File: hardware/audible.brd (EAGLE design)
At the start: 27.7 x 23.4 mm, 30 parts, among them IC1 LTC1966CMS8, J1 SQUALL_HEADER, J2 HIROSE-DF40C-10DP-0.4V, J3 HIROSE-DF40C-10DP-0.4V, J5 TC2030-JLINK-NL, Q1 FK3503010L, U1 MAX417ESA+, U2 MAX417ESA+

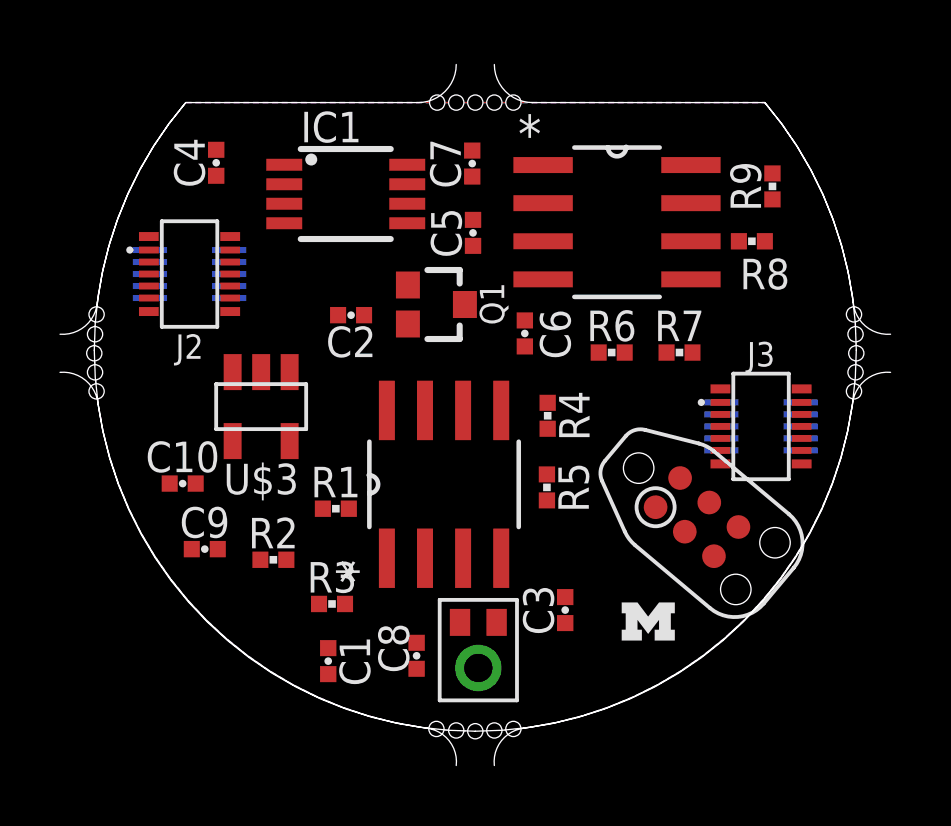
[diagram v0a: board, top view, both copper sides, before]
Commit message: almost routed
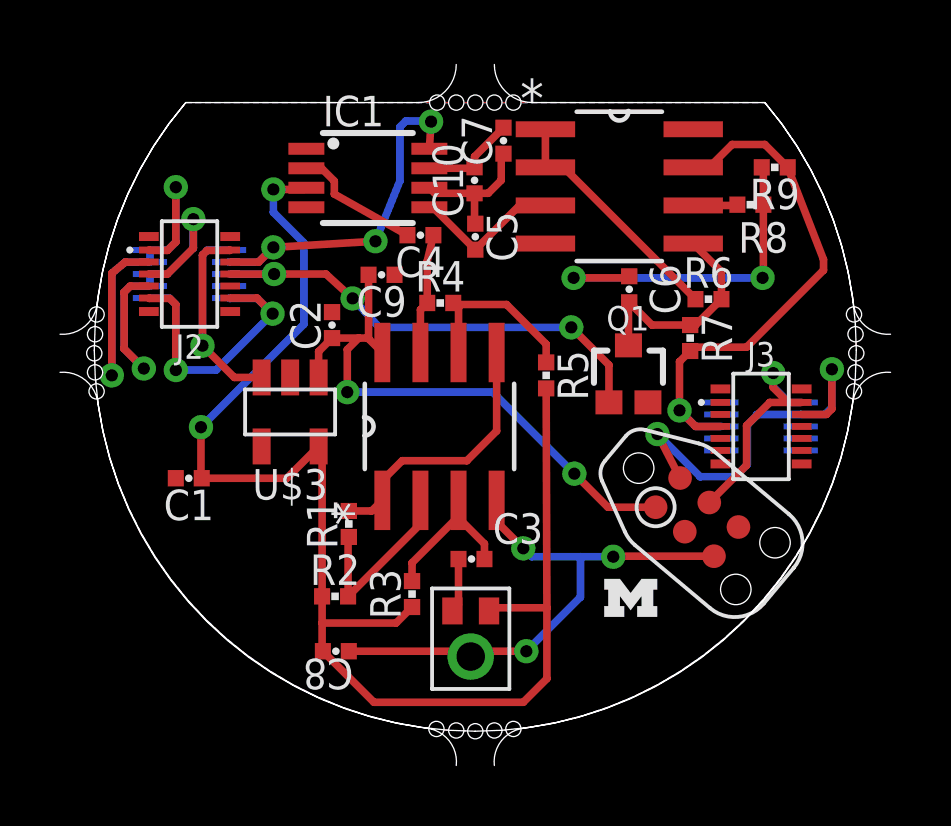
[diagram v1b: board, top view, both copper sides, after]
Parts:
- moved C10 14.0 mm to (24.1, 18.4), turned to 90 degrees
- moved C9 10.9 mm to (21.0, 15.2), turned to 180 degrees
- moved C1 7.67 mm to (14.6, 8.43), turned to 180 degrees
- moved C4 7.22 mm to (22.3, 16.5), turned to 180 degrees
- moved Q1 6.81 mm to (29.2, 11.9), turned to 0 degrees
- moved R4 5.19 mm to (23.0, 14.3), turned to 0 degrees
- moved C6 3.78 mm to (29.3, 14.7)
- moved R5 3.73 mm to (26.5, 11.9)
- moved R6 3.68 mm to (31.9, 14.4)
- moved C3 3.56 mm to (24.0, 5.74), turned to 0 degrees
- moved C8 2.70 mm to (19.5, 2.67), turned to 0 degrees
- moved R3 2.69 mm to (22.0, 4.57), turned to 90 degrees
- moved R2 2.39 mm to (19.5, 4.50)
- moved U1 1.94 mm to (22.9, 10.2)
- moved C7 1.29 mm to (25.1, 19.7)
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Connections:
- net A5: no longer J3.9
- net A6: no longer J3.7
- net MISO: no longer J3.8
- net MOSI: no longer J3.6
- net P25: no longer J2.8
- net SCL: no longer J3.3
- net SCLK: no longer J3.10
- net SDA: no longer J3.1
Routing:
- net GND: track 0.00 -> 48.6 mm, vias 0 -> 7
- net VREF: track 0.00 -> 47.2 mm, vias 0 -> 2
- net VCC: track 0.00 -> 38.4 mm, vias 0 -> 4
- net A7: track 0.00 -> 18.3 mm, vias 0 -> 1
- net P24: track 0.00 -> 16.6 mm, vias 0 -> 3
- net SWDIO/!RESET: track 0.00 -> 13.5 mm, vias 0 -> 2
- net 5V: track 0.00 -> 13.5 mm, vias 0 -> 2
- net P23: track 0.00 -> 12.7 mm, vias 0 -> 3
- net P22: track 0.00 -> 10.4 mm, vias 0 -> 1
- net MIC_AMP_1: track 0.00 -> 9.03 mm
- net RMS_BUF: track 0.00 -> 8.09 mm
- net SWDCLK: track 0.00 -> 8.00 mm, vias 0 -> 1
- net N$10: track 0.00 -> 7.44 mm
- net N$4: track 0.00 -> 6.19 mm
- net N$5: track 0.00 -> 6.00 mm
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
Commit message: routed
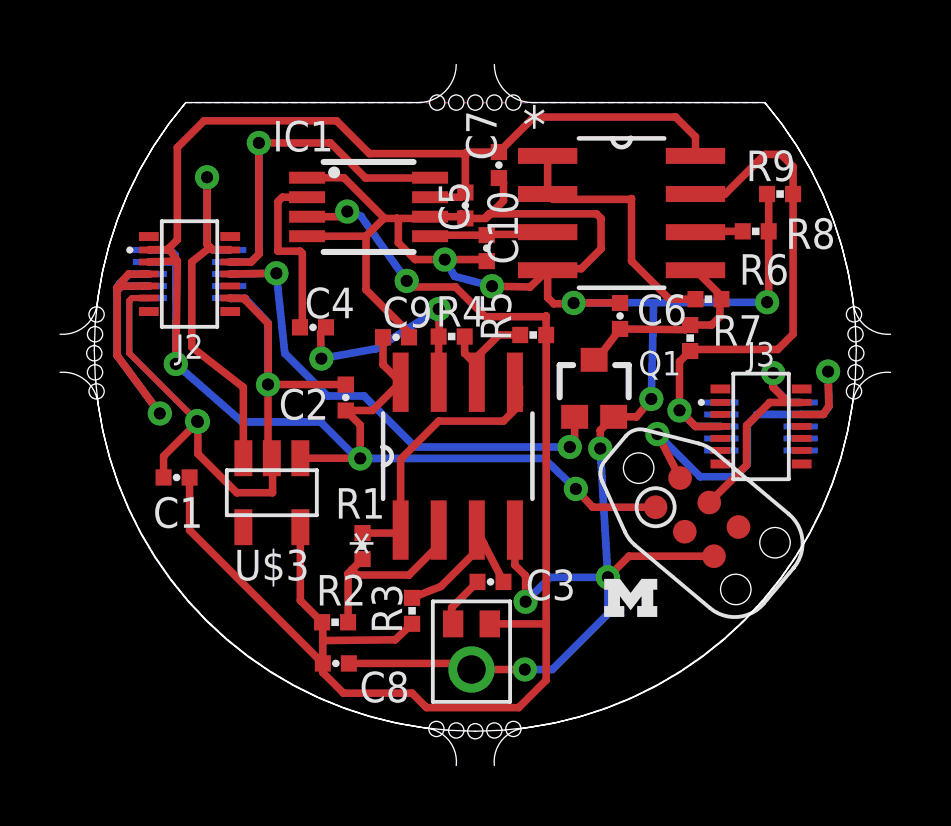
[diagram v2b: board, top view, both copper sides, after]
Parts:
- moved C4 4.72 mm to (18.7, 13.5)
- moved U$3 2.76 mm to (17.3, 7.95)
- moved C2 2.46 mm to (19.8, 11.1)
- moved C9 2.14 mm to (21.5, 13.1)
- moved R5 1.41 mm to (26.1, 13.2), turned to 0 degrees
- moved Q1 1.24 mm to (28.1, 11.4)
- moved R4 1.18 mm to (23.3, 13.2)
- moved U1 1.16 mm to (23.5, 9.17)
- moved C3 0.99 mm to (24.6, 4.98)
- moved IC1 0.97 mm to (20.6, 17.5)
- moved C6 0.94 mm to (29.0, 13.8)
- moved R8 0.91 mm to (33.5, 16.7)
- moved R9 0.91 mm to (34.3, 17.9)
- moved U2 0.89 mm to (29.0, 17.3)
- moved C10 0.89 mm to (23.8, 17.5)
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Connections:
- removed net A5: J1.B9
- removed net A6: J1.B7
- removed net MISO: J1.B8
- removed net MOSI: J1.B6
- removed net P25: J1.A8
- removed net SCL: J1.B3
- removed net SCLK: J1.B10
- removed net SDA: J1.B1
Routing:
- net GND: track 48.6 -> 105.1 mm, vias 7 -> 12
- net VCC: track 38.4 -> 62.3 mm, vias 4 -> 3
- net MIC_AMP_2: track 4.03 -> 8.24 mm, vias 0 -> 2
- net P22: track 10.4 -> 14.3 mm
- net P23: track 12.7 -> 15.8 mm, vias 3 -> 1
- net 5V: track 13.5 -> 16.0 mm, vias 2 -> 1
- net N$5: track 6.00 -> 3.66 mm
- net N$2: track 4.34 -> 6.02 mm
- net VREF: track 47.2 -> 48.6 mm
- net N$3: track 5.06 -> 3.95 mm
- net P24: track 16.6 -> 17.7 mm, vias 3 -> 2
- net RMS_BUF: track 8.09 -> 8.89 mm
- net N$10: track 7.44 -> 6.81 mm
